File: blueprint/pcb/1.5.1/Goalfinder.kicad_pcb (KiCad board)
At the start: 2 copper layers, 70 x 40.1 mm, 25 parts, among them J1 USB in, J2 USB-ESP, J3 GAIN, J4 LED Strip, J5 SW240 - Vcc/D0/GND, J6 VL53L0X-ToF Vcc/SDA/SCL/GND, Q1 IRLML2502, U1 ESP32 D1 Mini, U2 VL53L0X - ToF, U3 MAX98357A - Amplifier

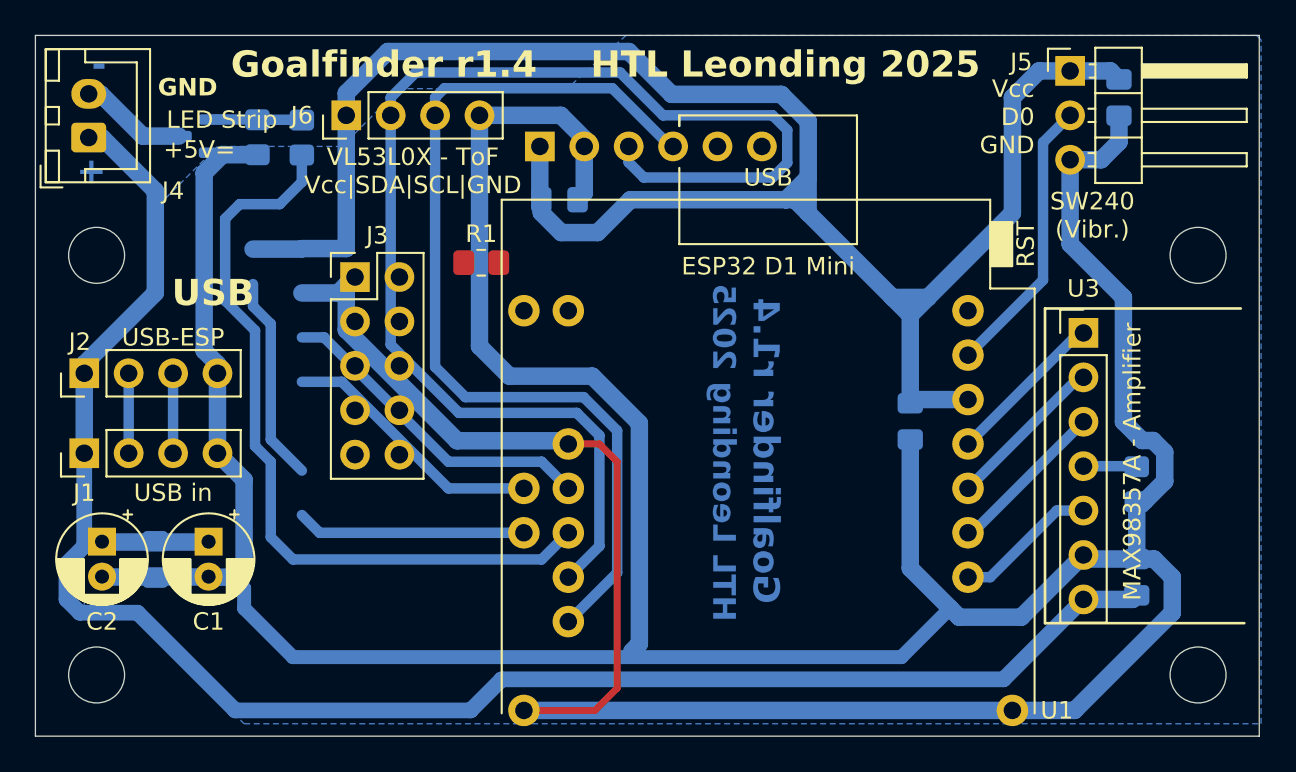
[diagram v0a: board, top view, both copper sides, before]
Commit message: Cleared PCB
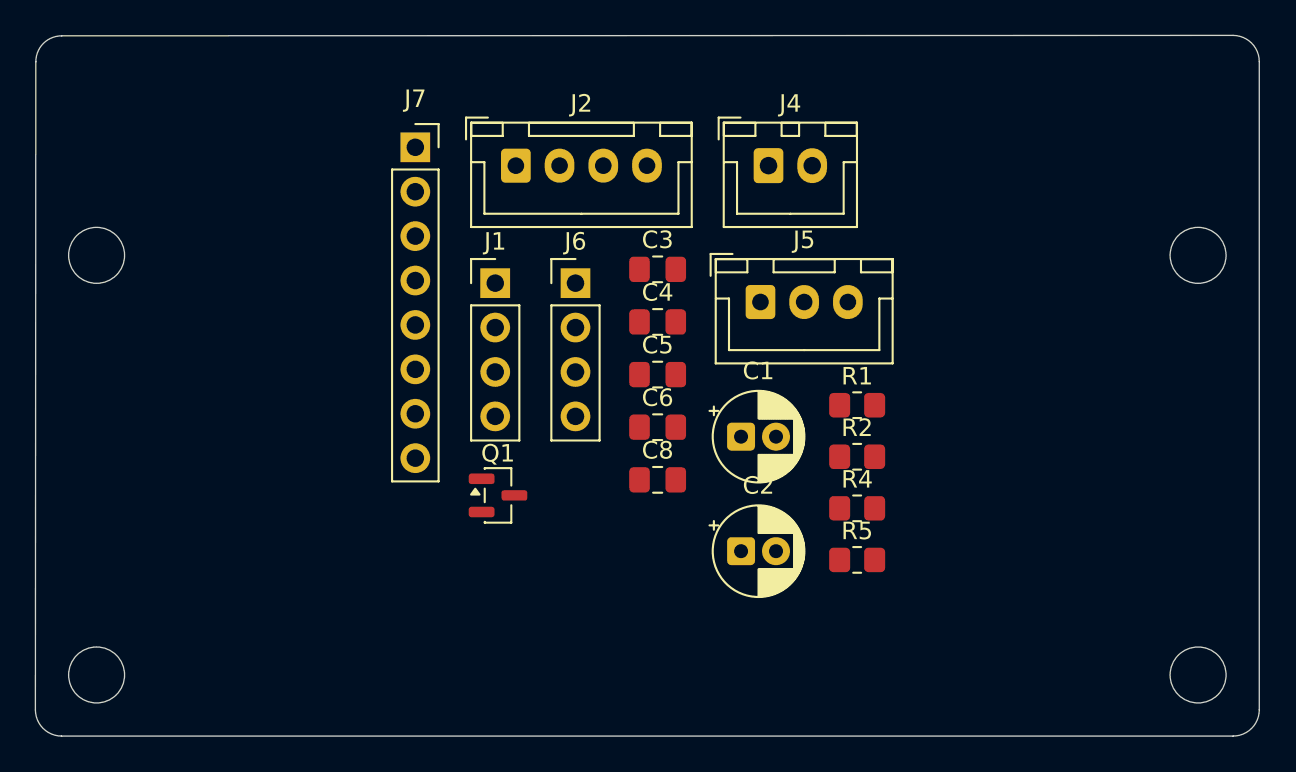
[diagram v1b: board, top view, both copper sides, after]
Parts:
- removed J3: GAIN, Connector_PinHeader_2.54mm:PinHeader_2x05_P2.54mm_Vertical
- removed U1: ESP32 D1 Mini, ESP32_D1_mini:ESP32_D1_mini
- removed U2: VL53L0X - ToF, Breakout_Boards:VL53L0X_Breakout_Board_vertical_flat
- removed U3: MAX98357A - Amplifier, Breakout_Boards:MAX98357A_Breakout_Board
- added J7: Conn_01x08_Pin, Connector_PinSocket_2.54mm:PinSocket_1x08_P2.54mm_Vertical, F.Cu at (136.7, 71.8)
- C3, C4, C5, C6, C8, Q1, R2, R4, R5: moved to F.Cu
- J2: footprint Connector_PinHeader_2.54mm:PinHeader_1x04_P2.54mm_Vertical -> Connector_JST:JST_XH_B4B-XH-A_1x04_P2.50mm_Vertical
- J5: footprint Connector_PinHeader_2.54mm:PinHeader_1x03_P2.54mm_Horizontal -> Connector_JST:JST_XH_B3B-XH-A_1x03_P2.50mm_Vertical
- moved R5 42.0 mm to (161.9, 95.4), turned to 0 degrees
- moved J4 38.9 mm to (156.9, 72.9), turned to 0 degrees
- moved R4 38.2 mm to (161.9, 92.5), turned to 0 degrees
- moved C2 36.6 mm to (155.3, 94.9), turned to 0 degrees
- moved C3 33.2 mm to (150.5, 78.8), turned to 0 degrees
- moved C4 31.0 mm to (150.5, 81.8), turned to 0 degrees
- moved C1 31.0 mm to (155.3, 88.4), turned to 0 degrees
- moved C5 30.8 mm to (150.5, 84.8), turned to 0 degrees
- moved J2 27.4 mm to (142.4, 72.9), turned to 0 degrees
- moved Q1 26.9 mm to (141.4, 91.7), turned to 0 degrees
- moved J1 25.4 mm to (141.2, 79.6), turned to 0 degrees
- moved R1 23.0 mm to (161.9, 86.6)
- moved J5 22.1 mm to (156.4, 80.7)
- moved J6 16.2 mm to (145.8, 79.6), turned to 0 degrees
- moved R2 16.1 mm to (161.9, 89.5), turned to 0 degrees
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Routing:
- net GND: track 268.1 -> 0.00 mm
- net 3V3: track 111.4 -> 0.00 mm
- net 5V: track 103.2 -> 0.00 mm
- net Net-(J6-Pin_2): track 74.3 -> 0.00 mm
- net Net-(J6-Pin_3): track 54.6 -> 0.00 mm
- net Net-(U1-IO_17/U2_TXC): track 44.3 -> 0.00 mm
- net unconnected-(U1-IO_16/U2_RX-Pad31): track 18.8 -> 0.00 mm
- net Net-(J5-Pin_2): track 16.1 -> 0.00 mm
- net unconnected-(U1-IO_04-Pad32): track 15.2 -> 0.00 mm
- net unconnected-(U1-IO_12/TDI-Pad30): track 13.1 -> 0.00 mm
- net (no net): track 11.8 -> 0.00 mm
- net Net-(U1-IO_23/MOSI): track 8.98 -> 0.00 mm
- net Net-(U1-IO_19/MISO): track 8.98 -> 0.00 mm
- net Net-(U1-IO_05/SS): track 8.98 -> 0.00 mm
- net Net-(U1-IO_18/CLK): track 8.18 -> 0.00 mm
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- removed copper zone on B.Cu, net GND
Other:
- outline, holes or cut-outs redrawn
- board text removed: "+"
- board text removed: "+5V="
- board text removed: "-"
- board text removed: "ESP32-D1 internal"
- board text removed: "GND"
- board text removed: "Goalfinder r1.4"
- board text removed: "HTL Leonding 2025"
- board text removed: "R2: max. gain (15dB) --: med. gain ( 9dB)"
- board text removed: "SW240 (Vibr.)"
- board text removed: "USB"
- board text removed: "VL53L0X - ToF Vcc|SDA|SCL|GND"
- board text removed: "Vcc D0 GND"
